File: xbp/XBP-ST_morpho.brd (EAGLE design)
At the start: 68.9 x 31.1 mm, 4 parts

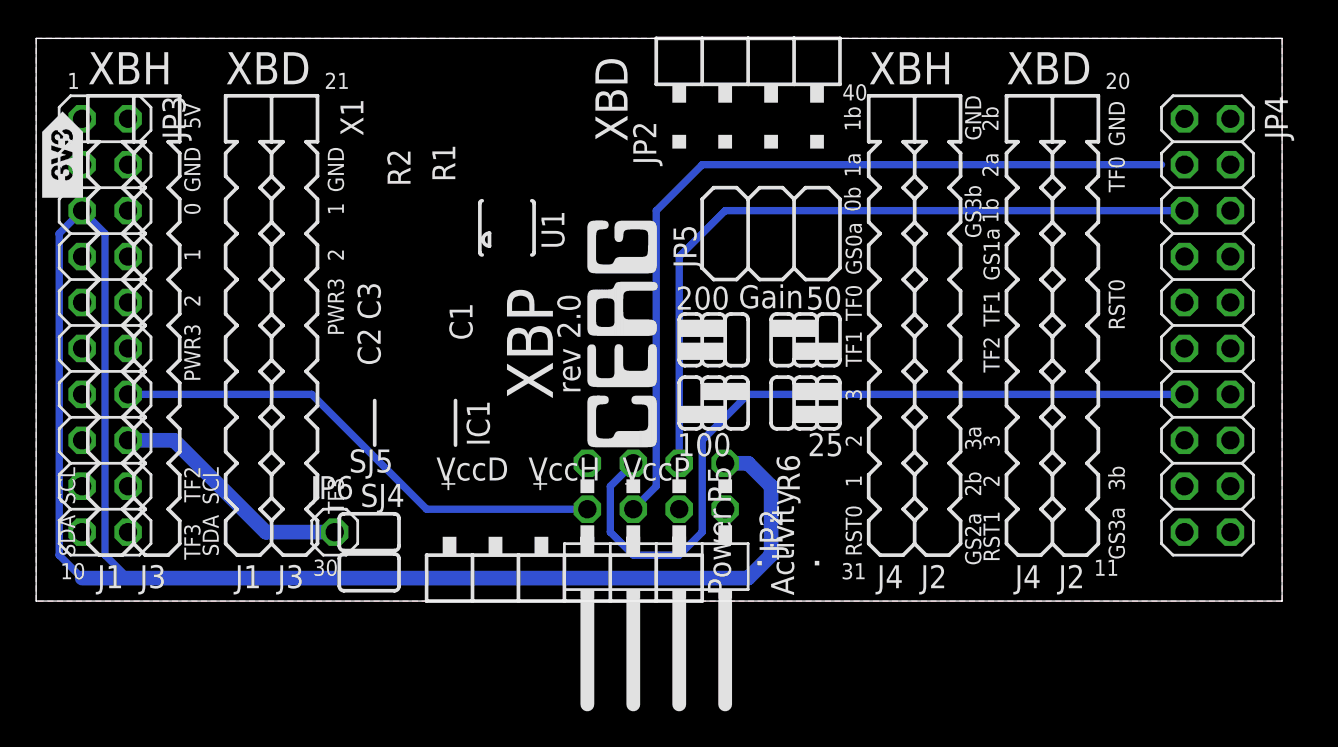
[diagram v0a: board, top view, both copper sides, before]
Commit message: XBX ST morpho Adapter version 1.0
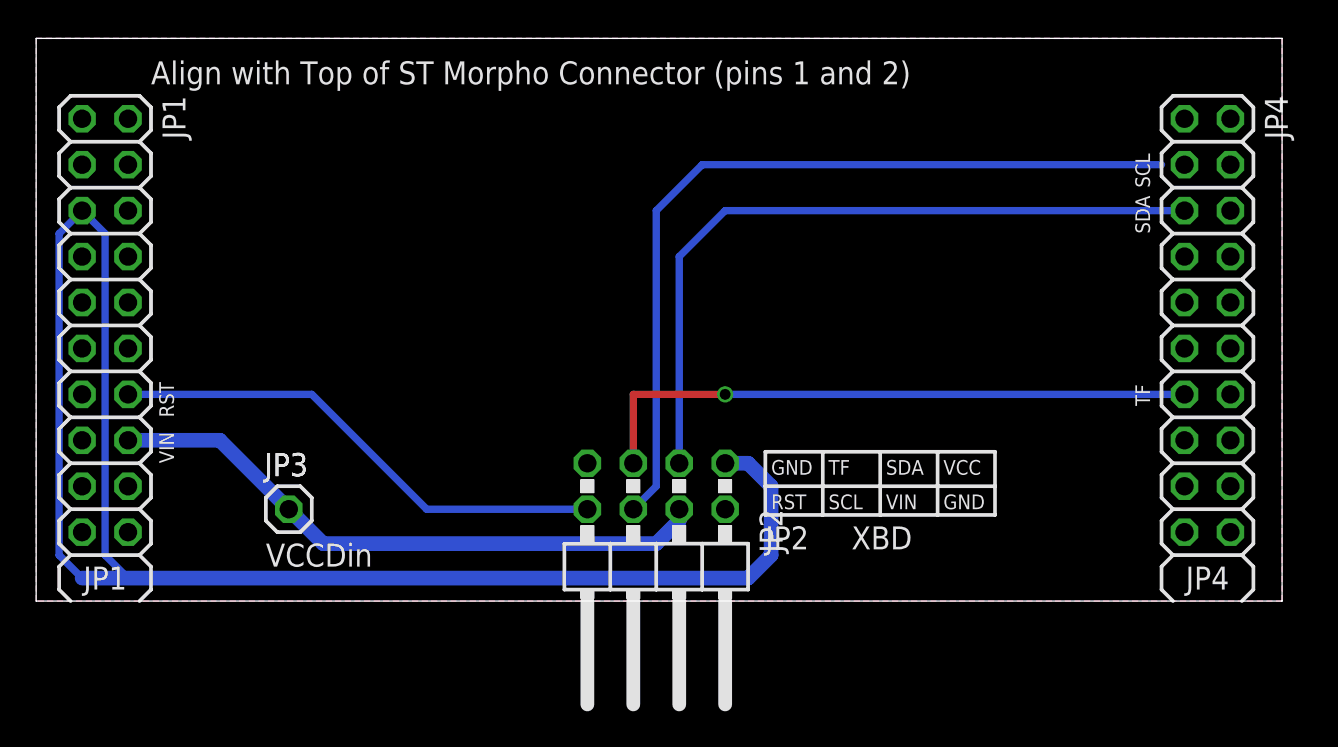
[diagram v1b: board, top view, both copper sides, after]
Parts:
- removed JP6: VCCDin, pinhead:1X01
- added JP1: (no value), pinhead:2X10
- JP3: value (none) -> VCCDin; device pinhead:2X10 -> pinhead:1X01
- moved JP3 14.4 mm to (14.0, 5.08), turned to 0 degrees
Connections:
- net GND: now also JP1.19, JP1.20, JP1.8, JP4.20; no longer JP3.8
- net N$6: now also JP1.16, JP2.4, JP3.1; no longer JP3.16, JP6.1
- net RSTD: now also JP1.14; no longer JP3.14
- net VCCD: now also JP1.5; no longer JP3.5
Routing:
- net N$6: track 13.5 -> 34.0 mm
- net TF0D: track 43.3 -> 34.3 mm, vias 0 -> 1
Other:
- board text added: "Align with Top of ST Morpho Connector (pins 1 and 2)"
- board text added: "JP1"
- board text added: "JP3"
- board text added: "JP4"
- board text added: "VCCDin"
- board text added: "VIN"
- board text added: "XXBX: XBP - ST morpho Adapter"
- board text added: "rev 1.0"
- board text removed: "+"
- board text removed: "0"
- board text removed: "0b"
- board text removed: "1"
- board text removed: "10"
- board text removed: "100"
- board text removed: "11"
- board text removed: "1a"
- board text removed: "1b"
- board text removed: "2"
- board text removed: "20"
- board text removed: "200"
- board text removed: "21"
- board text removed: "25"
- board text removed: "2a"
- board text removed: "2b"
- board text removed: "3"
- board text removed: "30"
- board text removed: "31"
- board text removed: "3a"
- board text removed: "3b"
- board text removed: "40"
- board text removed: "50"
- board text removed: "5V"
- board text removed: "Activity"
- board text removed: "C1"
- board text removed: "C2"
- board text removed: "C3"
- board text removed: "GS0a"
- board text removed: "GS1a"
- board text removed: "GS2a"
- board text removed: "GS3a"
- board text removed: "GS3b"
- board text removed: "Gain"
- board text removed: "IC1"
- board text removed: "J1"
- board text removed: "J2"
- board text removed: "J3"
- board text removed: "J4"
- board text removed: "JP5"
- board text removed: "PWR3"
- board text removed: "Power"
- board text removed: "Q1"
- board text removed: "Q2"
- board text removed: "Q3"
- board text removed: "Q4"
- board text removed: "Q5"
- board text removed: "Q6"
- board text removed: "Q7"
- board text removed: "Q8"
- board text removed: "R1"
- board text removed: "R10"
- board text removed: "R11"
- board text removed: "R12"
- board text removed: "R13"
- board text removed: "R2"
- board text removed: "R3"
- board text removed: "R4"
- board text removed: "R5"
- board text removed: "R6"
- board text removed: "R7"
- board text removed: "R8"
- board text removed: "R9"
- board text removed: "RST0"
- board text removed: "RST1"
- board text removed: "SJ1"
- board text removed: "SJ2"
- board text removed: "SJ3"
- board text removed: "SJ4"
- board text removed: "SJ5"
- board text removed: "TF0"
- board text removed: "TF1"
- board text removed: "TF2"
- board text removed: "TF3"
- board text removed: "U1"
- board text removed: "VccD"
- board text removed: "VccH"
- board text removed: "VccP"
- board text removed: "X1"
- board text removed: "XBH"
- board text removed: "XBP"
- board text removed: "rev 2.0"
